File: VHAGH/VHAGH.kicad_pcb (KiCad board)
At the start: 2 copper layers, 83 parts, among them IC1 MC9S08MP16xLC, J1 +12V, J10 Conn_01x03, J11 Conn_01x03, J12 TDS, J13 PH, J14 DHT11, J15 LV_Agua, J16 LDR_CON, J17 I2C, J18 UART, J19 PROGRM, J2 LED_BAR1, J3 LED_BAR2, J4 M1, J5 M2, J6 M3, J7 M4, J8 Conn_01x03, J9 Conn_01x03, K1 RLY1, K2 RLY2, K3 RLY3, K4 RLY4, Q1 IRF3205, Q2 IRF3205, SW1 SWDIP4, U1 AP63205WU, U2 MIC4427, U3 ULN2803A, U4 LM358, U5 LM358, U6 PC817, Y1 Crystal

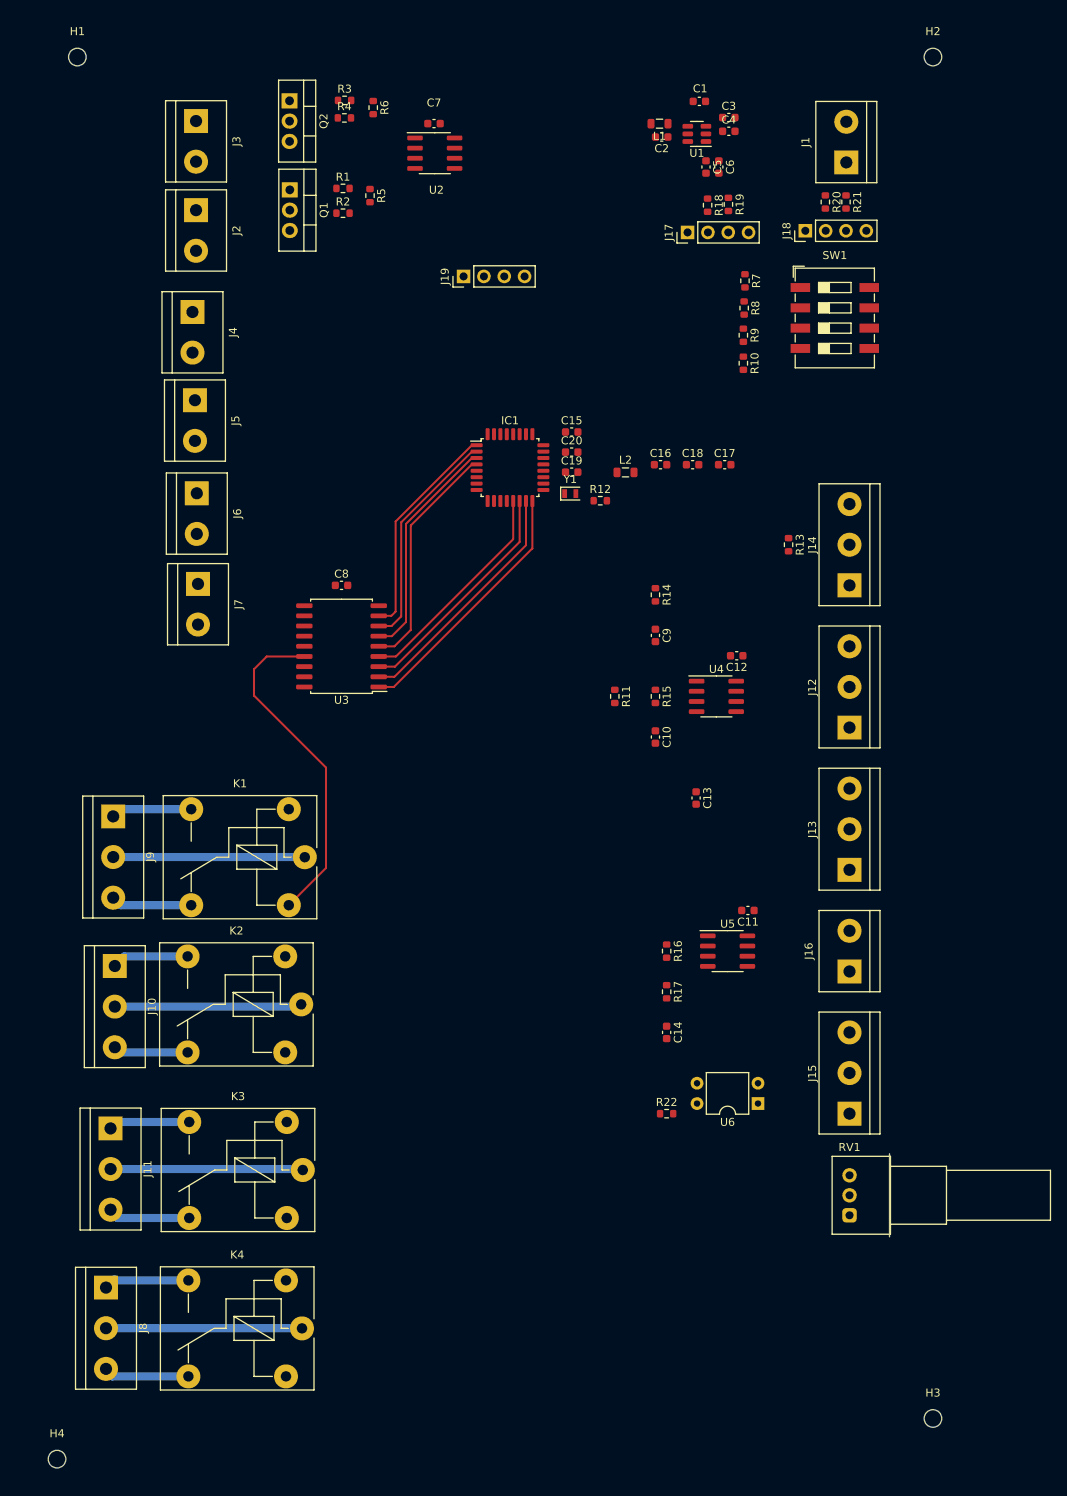
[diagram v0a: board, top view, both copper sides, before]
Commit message: modificado 7/22/22 6:05pm
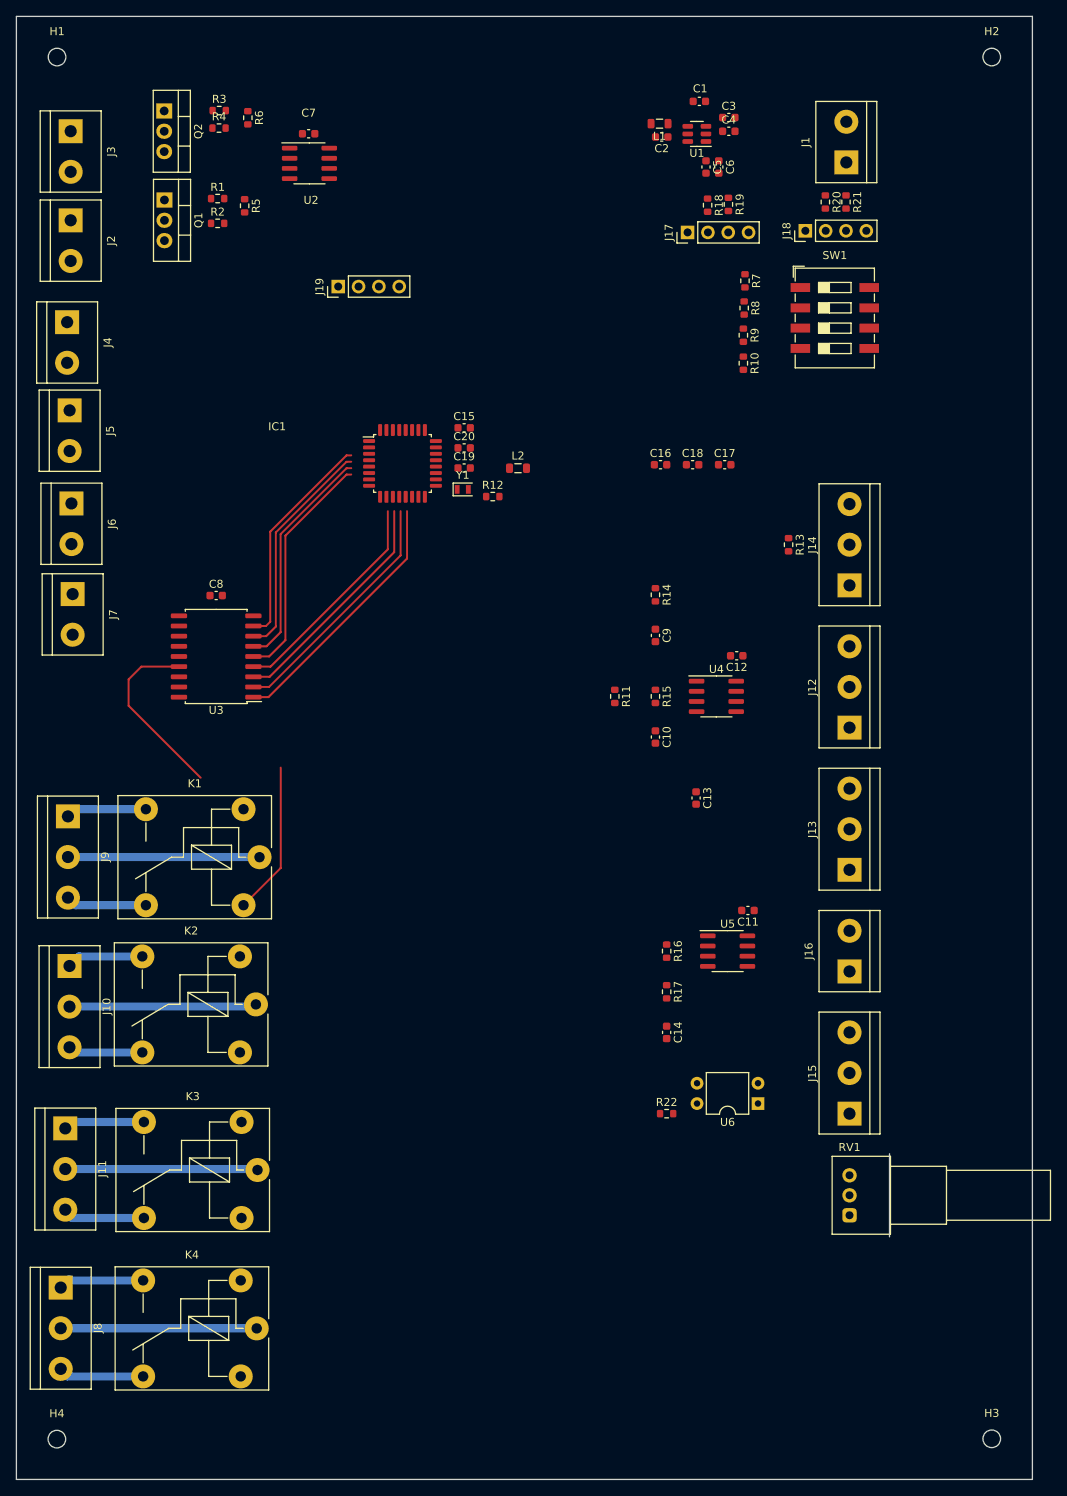
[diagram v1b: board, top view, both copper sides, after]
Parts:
- moved C7 15.7 mm to (49.2, 27.4)
- moved C8 15.7 mm to (37.7, 85.1)
- moved J2 15.7 mm to (19.5, 38.2)
- moved J3 15.7 mm to (19.5, 27.1)
- moved J4 15.7 mm to (19.0, 50.9)
- moved J5 15.7 mm to (19.4, 62.0)
- moved J6 15.7 mm to (19.6, 73.6)
- moved Q1 15.7 mm to (31.2, 35.6)
- moved R1 15.7 mm to (37.9, 35.5)
- moved R2 15.7 mm to (37.9, 38.6)
- moved R3 15.7 mm to (38.1, 24.5)
- moved R4 15.7 mm to (38.0, 26.7)
- moved R5 15.7 mm to (41.2, 36.4)
- moved U2 15.7 mm to (49.3, 31.1)
- moved U3 15.7 mm to (37.7, 92.7)
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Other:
- board outline added: 127 x 182.9 mm
